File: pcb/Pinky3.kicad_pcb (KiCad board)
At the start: 2 copper layers, 137 x 100.9 mm, 67 parts, among them J1 MJ-4PP-9, P1 i2c-pin, P2 i2c-pin, SW1 RESET_SW, SW10 SW_PUSH, SW11 SW_PUSH, SW12 SW_PUSH, SW13 SW_PUSH, SW14 SW_PUSH, SW15 SW_PUSH, SW16 SW_PUSH, SW17 SW_PUSH, SW18 SW_PUSH, SW19 SW_PUSH, SW2 SW_PUSH, SW20 SW_PUSH, SW21 SW_PUSH, SW22 SW_PUSH, SW23 SW_PUSH, SW24 SW_PUSH, SW25 SW_PUSH, SW26 SW_PUSH, SW3 SW_PUSH, SW4 SW_PUSH, SW5 SW_PUSH, SW6 SW_PUSH, SW7 SW_PUSH, SW8 SW_PUSH, SW9 SW_PUSH, U1 ProMicro

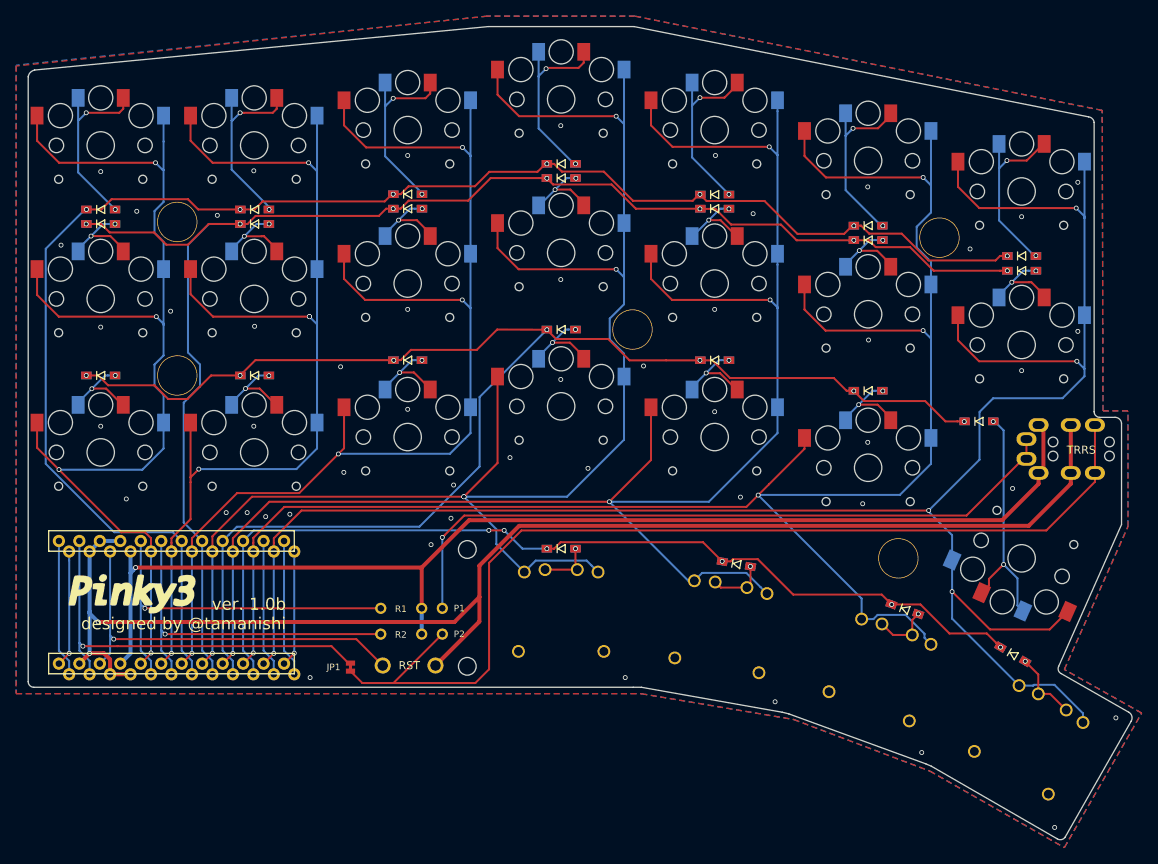
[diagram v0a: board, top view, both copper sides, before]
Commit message: merge flatten files
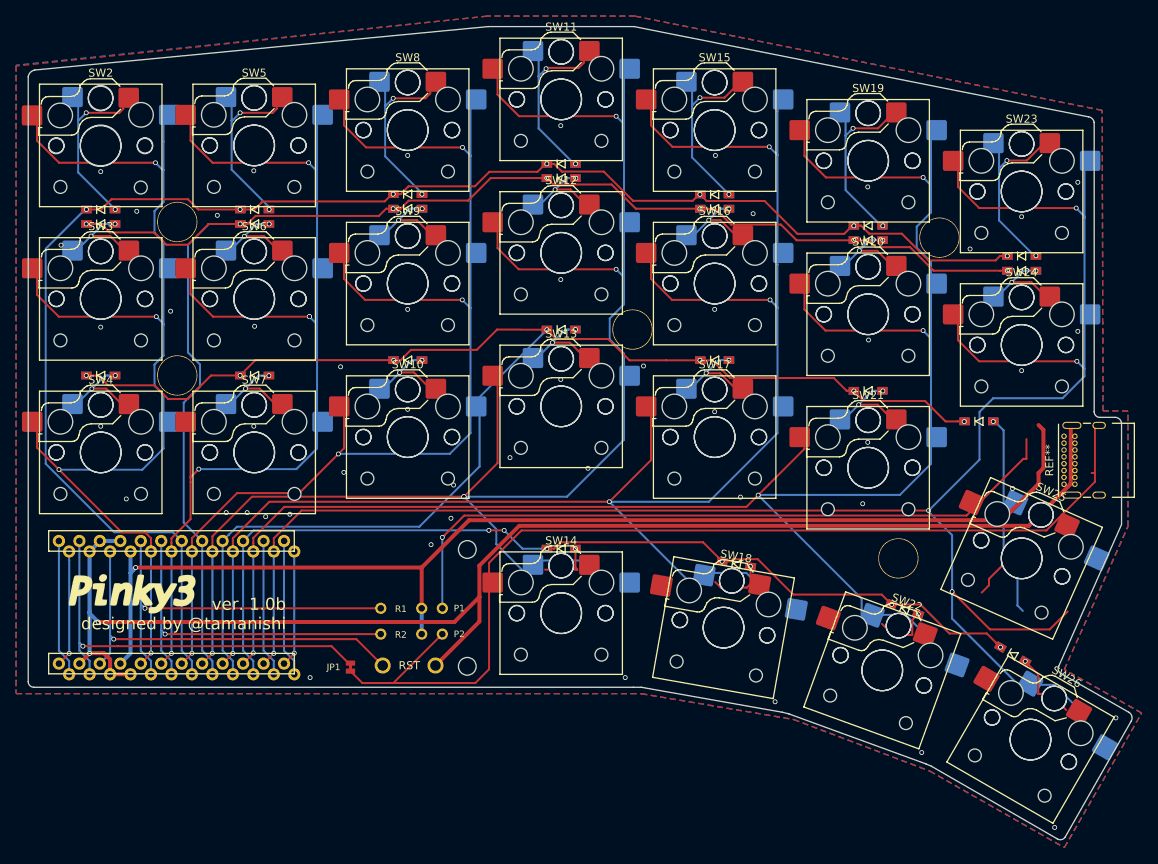
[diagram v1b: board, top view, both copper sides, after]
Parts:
- removed J1: MJ-4PP-9, kbd:MJ-4PP-9
- added REF**: USB_C_Receptacle_GCT_USB4085, Connector_USB:USB_C_Receptacle_GCT_USB4085, F.Cu at (169.6, 111.1)
- added SW10: SW_PUSH, Switch_Keyboard_Hotswap_Kailh:SW_Hotswap_Kailh_Choc_V1V2_1.00u, B.Cu at (88.1, 105.2)
- added SW11: SW_PUSH, Switch_Keyboard_Hotswap_Kailh:SW_Hotswap_Kailh_Choc_V1V2_1.00u, B.Cu at (107.2, 63.3)
- added SW12: SW_PUSH, Switch_Keyboard_Hotswap_Kailh:SW_Hotswap_Kailh_Choc_V1V2_1.00u, B.Cu at (107.2, 82.4)
- added SW13: SW_PUSH, Switch_Keyboard_Hotswap_Kailh:SW_Hotswap_Kailh_Choc_V1V2_1.00u, B.Cu at (107.2, 101.4)
- added SW14: SW_PUSH, Switch_Keyboard_Hotswap_Kailh:SW_Hotswap_Kailh_Choc_V1V2_1.00u, B.Cu at (107.2, 127.1)
- added SW15: SW_PUSH, Switch_Keyboard_Hotswap_Kailh:SW_Hotswap_Kailh_Choc_V1V2_1.00u, B.Cu at (126.2, 67.1)
- added SW16: SW_PUSH, Switch_Keyboard_Hotswap_Kailh:SW_Hotswap_Kailh_Choc_V1V2_1.00u, B.Cu at (126.2, 86.2)
- added SW17: SW_PUSH, Switch_Keyboard_Hotswap_Kailh:SW_Hotswap_Kailh_Choc_V1V2_1.00u, B.Cu at (126.2, 105.2)
- added SW18: SW_PUSH, Switch_Keyboard_Hotswap_Kailh:SW_Hotswap_Kailh_Choc_V1V2_1.00u, B.Cu at (127.3, 128.9)
- added SW19: SW_PUSH, Switch_Keyboard_Hotswap_Kailh:SW_Hotswap_Kailh_Choc_V1V2_1.00u, B.Cu at (145.2, 71.0)
- added SW2: SW_PUSH, Switch_Keyboard_Hotswap_Kailh:SW_Hotswap_Kailh_Choc_V1V2_1.00u, B.Cu at (50.0, 69.1)
- added SW20: SW_PUSH, Switch_Keyboard_Hotswap_Kailh:SW_Hotswap_Kailh_Choc_V1V2_1.00u, B.Cu at (145.2, 90.0)
- added SW21: SW_PUSH, Switch_Keyboard_Hotswap_Kailh:SW_Hotswap_Kailh_Choc_V1V2_1.00u, B.Cu at (145.2, 109.1)
- added SW22: SW_PUSH, Switch_Keyboard_Hotswap_Kailh:SW_Hotswap_Kailh_Choc_V1V2_1.00u, B.Cu at (147.0, 134.2)
- added SW23: SW_PUSH, Switch_Keyboard_Hotswap_Kailh:SW_Hotswap_Kailh_Choc_V1V2_1.00u, B.Cu at (164.3, 74.8)
- added SW24: SW_PUSH, Switch_Keyboard_Hotswap_Kailh:SW_Hotswap_Kailh_Choc_V1V2_1.00u, B.Cu at (164.3, 93.8)
- added SW25: SW_PUSH, Switch_Keyboard_Hotswap_Kailh:SW_Hotswap_Kailh_Choc_V1V2_1.00u, B.Cu at (164.3, 120.3)
- added SW26: SW_PUSH, Switch_Keyboard_Hotswap_Kailh:SW_Hotswap_Kailh_Choc_V1V2_1.00u, B.Cu at (165.4, 142.8)
- added SW3: SW_PUSH, Switch_Keyboard_Hotswap_Kailh:SW_Hotswap_Kailh_Choc_V1V2_1.00u, B.Cu at (50.0, 88.1)
- added SW4: SW_PUSH, Switch_Keyboard_Hotswap_Kailh:SW_Hotswap_Kailh_Choc_V1V2_1.00u, B.Cu at (50.0, 107.2)
- added SW5: SW_PUSH, Switch_Keyboard_Hotswap_Kailh:SW_Hotswap_Kailh_Choc_V1V2_1.00u, B.Cu at (69.0, 69.1)
- added SW6: SW_PUSH, Switch_Keyboard_Hotswap_Kailh:SW_Hotswap_Kailh_Choc_V1V2_1.00u, B.Cu at (69.0, 88.1)
- added SW7: SW_PUSH, Switch_Keyboard_Hotswap_Kailh:SW_Hotswap_Kailh_Choc_V1V2_1.00u, B.Cu at (69.0, 107.2)
- added SW8: SW_PUSH, Switch_Keyboard_Hotswap_Kailh:SW_Hotswap_Kailh_Choc_V1V2_1.00u, B.Cu at (88.1, 67.1)
- added SW9: SW_PUSH, Switch_Keyboard_Hotswap_Kailh:SW_Hotswap_Kailh_Choc_V1V2_1.00u, B.Cu at (88.1, 86.2)
- SW10, SW11, SW12, SW13, SW15, SW16, SW17, SW19, SW2, SW20, SW21, SW23, SW24, SW25, SW3, SW4, SW5, SW6, SW7, SW8, SW9: footprint lib:Choc_Hotswap -> Switch_Keyboard_Hotswap_Kailh:SW_Hotswap_Kailh_Choc_V1V2_1.00u
- SW14, SW18, SW22, SW26: footprint lib:kailh_low_choc -> Switch_Keyboard_Hotswap_Kailh:SW_Hotswap_Kailh_Choc_V1V2_1.00u
- turned SW14 to 0 degrees
- turned SW18 to -10 degrees
- turned SW22 to -20 degrees
- turned SW25 to -24 degrees
- turned SW26 to -30 degrees
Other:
- net class Default removed
